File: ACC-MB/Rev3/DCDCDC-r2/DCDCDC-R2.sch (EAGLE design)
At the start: 38 parts, among them P1330-102H 39uH

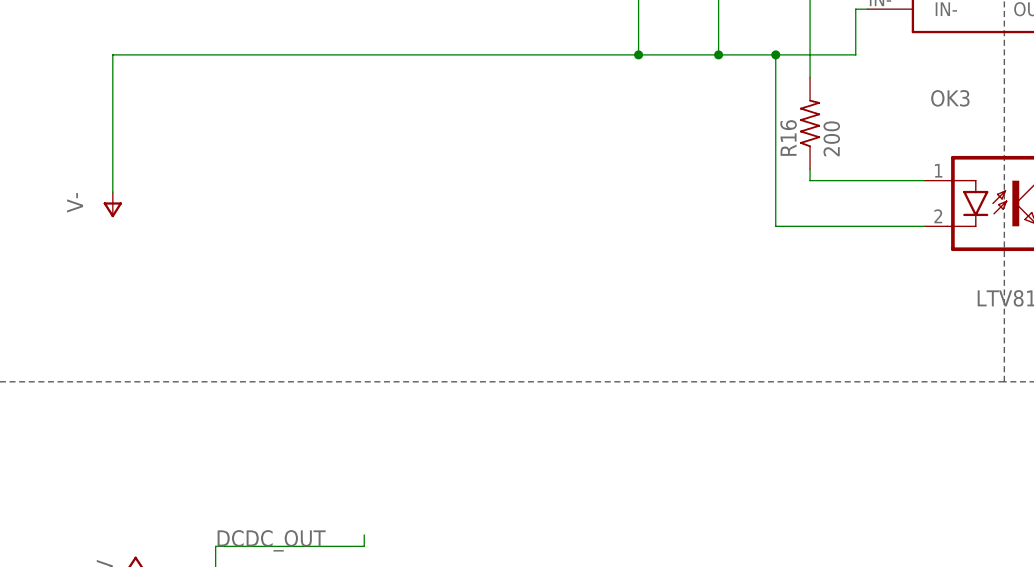
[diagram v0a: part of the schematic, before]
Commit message: d
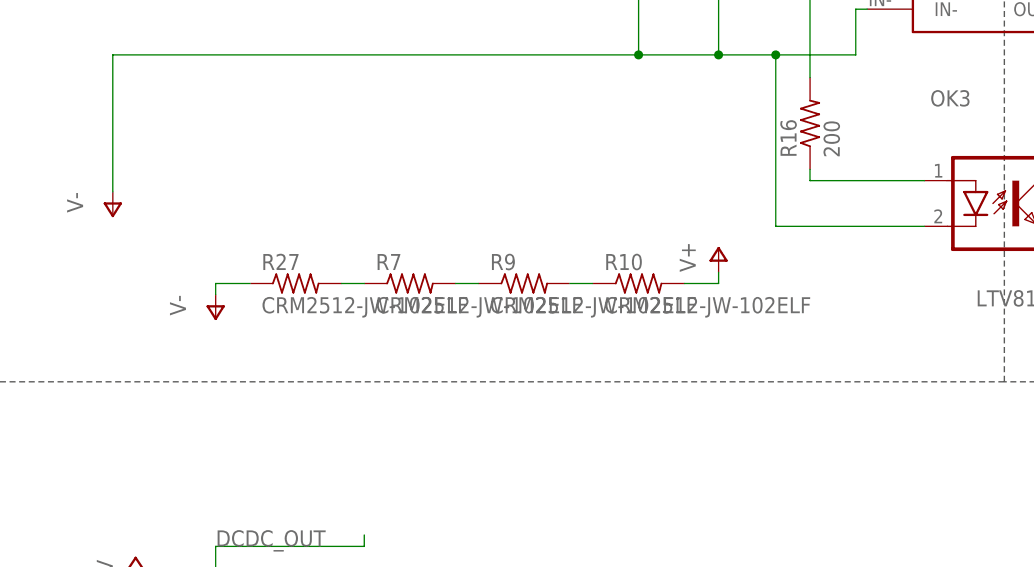
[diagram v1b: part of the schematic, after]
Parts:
- added R10, R27, R7, R9: CRM2512-JW-102ELF, ACC-MB-R0:R-US_R2512
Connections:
- new net N$12: R27.2, R7.1
- new net N$13: R7.2, R9.1
- new net N$14: R10.1, R9.2
- net V+: now also R10.2
- net V-: now also R27.1
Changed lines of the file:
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@@
 <part name="GND8" library="ACC-MB-R0" library_urn="urn:adsk.eagle:library:13208985" deviceset="GND" device=""/>
 <part name="U$13" library="ACC-MB-R0" library_urn="urn:adsk.eagle:library:13208985" deviceset="39-28-1103" device="" package3d_urn="urn:adsk.eagle:package:14745616/3"/>
-<part name="U$9" library="ACC-MB-R0" library_urn="urn:adsk.eagle:library:13208985" deviceset="15-24-6100" device="" package3d_urn="urn:adsk.eagle:package:14396594/2"/>
-<part name="U$10" library="ACC-MB-R0" library_urn="urn:adsk.eagle:library:13208985" deviceset="15-24-6100" device="" package3d_urn="urn:adsk.eagle:package:14396594/2"/>
+<part name="U$9" library="ACC-MB-R0" library_urn="urn:adsk.eagle:library:13208985" deviceset="15-24-6100" device="" package3d_urn="urn:adsk.eagle:package:14396594/3"/>
+<part name="U$10" library="ACC-MB-R0" library_urn="urn:adsk.eagle:library:13208985" deviceset="15-24-6100" device="" package3d_urn="urn:adsk.eagle:package:14396594/3"/>
 <part name="U$18" library="ACC-MB-R0" library_urn="urn:adsk.eagle:library:13208985" deviceset="SANACE40" device="" package3d_urn="urn:adsk.eagle:package:15010781/2" value="9GAX0412P3S0031"/>
 <part name="U$12" library="ACC-MB-R0" library_urn="urn:adsk.eagle:library:13208985" deviceset="VICOR_HEATSINK_DOUBLE" device="" package3d_urn="urn:adsk.eagle:package:15094638/2"/>
@@
 <part name="U$20" library="ACC-MB-R0" library_urn="urn:adsk.eagle:library:13208985" deviceset="BENDER_IRR155" device="" package3d_urn="urn:adsk.eagle:package:14400200/2"/>
 <part name="U$11" library="ACC-MB-R0" library_urn="urn:adsk.eagle:library:13208985" deviceset="0100-020" device=""/>
+<part name="R27" library="ACC-MB-R0" library_urn="urn:adsk.eagle:library:13208985" deviceset="R-US_" device="R2512" package3d_urn="urn:adsk.eagle:package:13209595/1" value="CRM2512-JW-102ELF"/>
+<part name="R7" library="ACC-MB-R0" library_urn="urn:adsk.eagle:library:13208985" deviceset="R-US_" device="R2512" package3d_urn="urn:adsk.eagle:package:13209595/1" value="CRM2512-JW-102ELF"/>
+<part name="R9" library="ACC-MB-R0" library_urn="urn:adsk.eagle:library:13208985" deviceset="R-US_" device="R2512" package3d_urn="urn:adsk.eagle:package:13209595/1" value="CRM2512-JW-102ELF"/>
+<part name="R10" library="ACC-MB-R0" library_urn="urn:adsk.eagle:library:13208985" deviceset="R-US_" device="R2512" package3d_urn="urn:adsk.eagle:package:13209595/1" value="CRM2512-JW-102ELF"/>
+<part name="P-3" library="ACC-MB-R0" library_urn="urn:adsk.eagle:library:13324935" deviceset="V-" device=""/>
+<part name="P+8" library="ACC-MB-R0" library_urn="urn:adsk.eagle:library:13324935" deviceset="V+" device=""/>
 </parts>
 <sheets>
@@
 <attribute name="VALUE" x="29.21" y="210.439" size="1.778" layer="96"/>
 </instance>
+<instance part="R27" gate="G$1" x="36.83" y="171.45" smashed="yes">
+<attribute name="NAME" x="33.02" y="172.9486" size="1.778" layer="95"/>
+<attribute name="VALUE" x="33.02" y="168.148" size="1.778" layer="96"/>
+</instance>
+<instance part="R7" gate="G$1" x="49.53" y="171.45" smashed="yes">
+<attribute name="NAME" x="45.72" y="172.9486" size="1.778" layer="95"/>
+<attribute name="VALUE" x="45.72" y="168.148" size="1.778" layer="96"/>
+</instance>
+<instance part="R9" gate="G$1" x="62.23" y="171.45" smashed="yes">
+<attribute name="NAME" x="58.42" y="172.9486" size="1.778" layer="95"/>
+<attribute name="VALUE" x="58.42" y="168.148" size="1.778" layer="96"/>
+</instance>
+<instance part="R10" gate="G$1" x="74.93" y="171.45" smashed="yes">
+<attribute name="NAME" x="71.12" y="172.9486" size="1.778" layer="95"/>
+<attribute name="VALUE" x="71.12" y="168.148" size="1.778" layer="96"/>
+</instance>
+<instance part="P-3" gate="1" x="27.94" y="167.64" smashed="yes">
+<attribute name="VALUE" x="22.86" y="170.18" size="1.778" layer="96" rot="R270"/>
+</instance>
+<instance part="P+8" gate="1" x="83.82" y="175.26" smashed="yes">
+<attribute name="VALUE" x="81.28" y="172.72" size="1.778" layer="96" rot="R90"/>
+</instance>
 </instances>
 <busses>
@@
 <pinref part="U$9" gate="G$1" pin="4"/>
 <wire x1="171.45" y1="99.06" x2="168.91" y2="99.06" width="0.1524" layer="91"/>
+</segment>
+<segment>
+<pinref part="R10" gate="G$1" pin="2"/>
+<wire x1="80.01" y1="171.45" x2="83.82" y2="171.45" width="0.1524" layer="91"/>
+<pinref part="P+8" gate="1" pin="V+"/>
+<wire x1="83.82" y1="171.45" x2="83.82" y2="172.72" width="0.1524" layer="91"/>
 </segment>
 </net>
@@
 <wire x1="176.53" y1="111.76" x2="179.07" y2="111.76" width="0.1524" layer="91"/>
 <junction x="179.07" y="111.76"/>
+</segment>
+<segment>
+<pinref part="R27" gate="G$1" pin="1"/>
+<wire x1="31.75" y1="171.45" x2="27.94" y2="171.45" width="0.1524" layer="91"/>
+<pinref part="P-3" gate="1" pin="V-"/>
+<wire x1="27.94" y1="170.18" x2="27.94" y2="171.45" width="0.1524" layer="91"/>
 </segment>
 </net>
@@
 </segment>
 </net>
+<net name="N$12" class="0">
+<segment>
+<pinref part="R27" gate="G$1" pin="2"/>
+<pinref part="R7" gate="G$1" pin="1"/>
+<wire x1="41.91" y1="171.45" x2="44.45" y2="171.45" width="0.1524" layer="91"/>
+</segment>
+</net>
+<net name="N$13" class="0">
+<segment>
+<pinref part="R7" gate="G$1" pin="2"/>
+<pinref part="R9" gate="G$1" pin="1"/>
+<wire x1="54.61" y1="171.45" x2="57.15" y2="171.45" width="0.1524" layer="91"/>
+</segment>
+</net>
+<net name="N$14" class="0">
+<segment>
+<pinref part="R9" gate="G$1" pin="2"/>
+<pinref part="R10" gate="G$1" pin="1"/>
+<wire x1="67.31" y1="171.45" x2="69.85" y2="171.45" width="0.1524" layer="91"/>
+</segment>
+</net>
